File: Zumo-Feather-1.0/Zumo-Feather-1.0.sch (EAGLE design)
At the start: 8 parts, among them U1 BRD-ARDUINOR3-DIMENSION

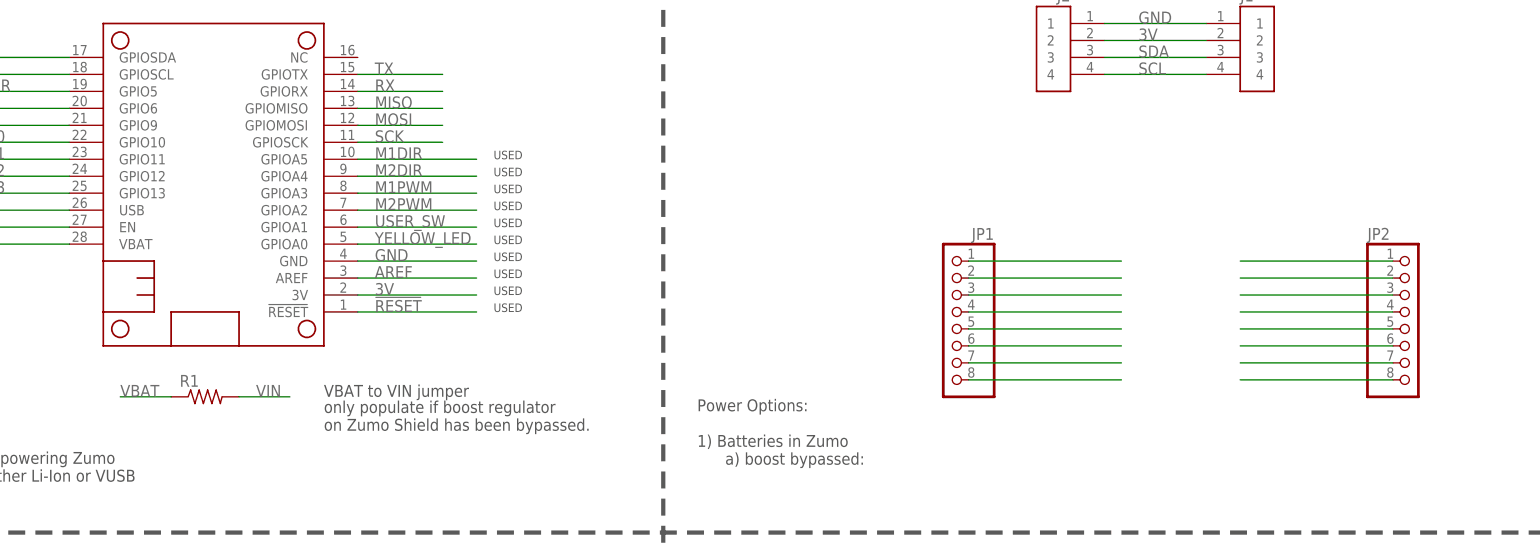
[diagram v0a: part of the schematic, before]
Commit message: Updated schematic
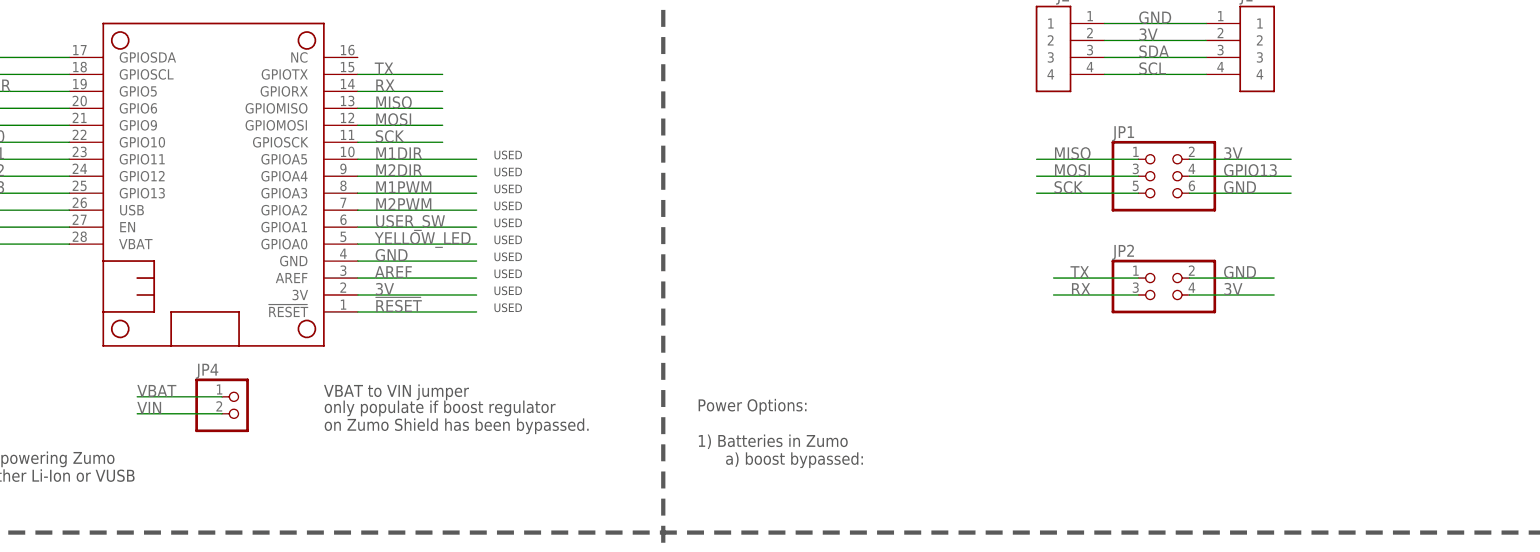
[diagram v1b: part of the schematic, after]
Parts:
- removed R1: (no value), RLC:R-US_R0805
- added JP4: (no value), pinhead:PINHD-1X2
- JP1: device pinhead:PINHD-1X8 -> pinhead:PINHD-2X3
- JP2: device pinhead:PINHD-1X8 -> pinhead:PINHD-2X2
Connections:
- removed net N$10: JP2.6
- removed net N$11: JP2.7
- removed net N$12: JP2.8
- removed net N$13: JP1.1
- removed net N$14: JP1.2
- removed net N$15: JP1.3
- removed net N$16: JP1.4
- removed net N$17: JP1.5
- removed net N$18: JP1.6
- removed net N$19: JP1.7
- removed net N$20: JP1.8
- removed net N$5: JP2.1
- removed net N$6: JP2.2
- removed net N$7: JP2.3
- removed net N$8: JP2.4
- removed net N$9: JP2.5
- net 3V: now also JP1.2, JP2.4
- net GND: now also JP1.6, JP2.2
- net GPIO13: now also JP1.4
- net MISO: now also JP1.1
- net MOSI: now also JP1.3
- net RX: now also JP2.3
- net SCK: now also JP1.5
- net TX: now also JP2.1
- net VBAT: now also JP4.1; no longer R1.1
- net VIN: now also JP4.2; no longer R1.2
